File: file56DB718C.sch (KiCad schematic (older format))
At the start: 1 part, among them U4 SX1276

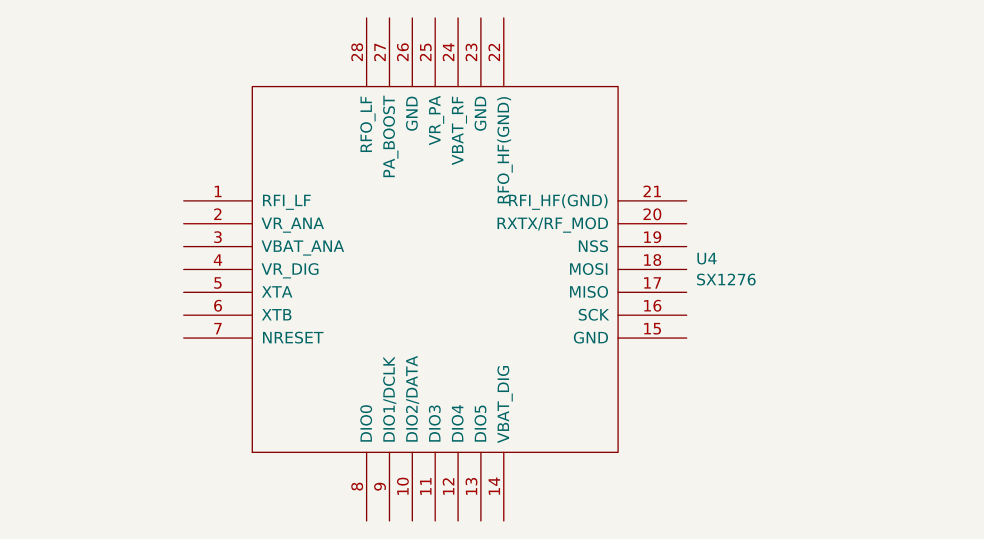
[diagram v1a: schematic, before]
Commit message: started layout, completed schematic
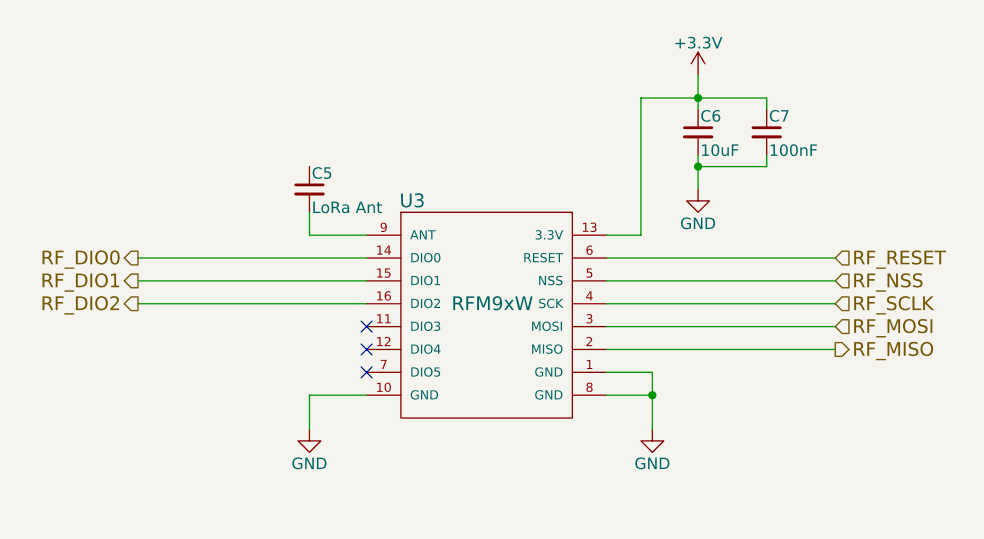
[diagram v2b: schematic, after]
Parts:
- removed U4: SX1276, Housings_DFN_QFN:QFN-28-1EP_6x6mm_Pitch0.65mm, symbol SX1276
- added C5: LoRa Ant, symbol C_Small
- added C6: 10uF, symbol C_Small
- added C7: 100nF, symbol C_Small
- added U3: RFM9xW, RocketScreamKicadLibrary:RFM9xW, symbol RFM9xW
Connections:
- new net: C5.2, U3.9 (ANT)
- new net +3V3: C6.1, C7.1, U3.13 (3.3V)
- new net GND: C6.2, C7.2, U3.1 (GND), U3.10 (GND), U3.8 (GND)
- new net RF_DIO0: U3.14 (DIO0)
- new net RF_DIO1: U3.15 (DIO1)
- new net RF_DIO2: U3.16 (DIO2)
- new net RF_MISO: U3.2 (MISO)
- new net RF_MOSI: U3.3 (MOSI)
- new net RF_NSS: U3.5 (NSS)
- new net RF_RESET: U3.6 (RESET)
- new net RF_SCLK: U3.4 (SCK)
- no-connect marks 0 -> 3
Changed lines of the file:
@@
 LIBS:mpu-9250
 LIBS:SAMD21E17A
+LIBS:miniultrapro
+LIBS:texas-instruments
 LIBS:lorawan_gps-cache
 EELAYER 25 0
@@
 $Descr A4 11693 8268
 encoding utf-8
-Sheet 5 7
+Sheet 4 7
 Title ""
 Date ""
@@
 $EndDescr
 $Comp
-L SX1276 U4
-U 1 1 56DB7573
-P 5400 3050
-F 0 "U4" H 6541 3096 50  0000 L CNN
-F 1 "SX1276" H 6541 3004 50  0000 L CNN
-F 2 "Housings_DFN_QFN:QFN-28-1EP_6x6mm_Pitch0.65mm" H 5400 3050 50  0001 C CNN
-F 3 "DOCUMENTATION" H 5400 3050 50  0001 C CNN
-	1    5400 3050
+L RFM9xW U3
+U 1 1 56EAE0A1
+P 5650 3250
+F 0 "U3" H 5300 3750 60  0000 C CNN
+F 1 "RFM9xW" H 5650 3300 60  0000 C CNN
+F 2 "RocketScreamKicadLibrary:RFM9xW" H 5650 2750 60  0001 C CNN
+F 3 "" H 5650 3550 60  0000 C CNN
+	1    5650 3250
 	1    0    0    -1
 $EndComp
+NoConn ~ 5100 3300
+NoConn ~ 5100 3400
+NoConn ~ 5100 3500
+$Comp
+L GND #PWR8
+U 1 1 56EAE13D
+P 4850 3750
+F 0 "#PWR8" H 4850 3500 50  0001 C CNN
+F 1 "GND" H 4850 3600 50  0000 C CNN
+F 2 "" H 4850 3750 50  0000 C CNN
+F 3 "" H 4850 3750 50  0000 C CNN
+	1    4850 3750
+	1    0    0    -1
+$EndComp
+$Comp
+L GND #PWR9
+U 1 1 56EAE153
+P 6350 3750
+F 0 "#PWR9" H 6350 3500 50  0001 C CNN
+F 1 "GND" H 6350 3600 50  0000 C CNN
+F 2 "" H 6350 3750 50  0000 C CNN
+F 3 "" H 6350 3750 50  0000 C CNN
+	1    6350 3750
+	1    0    0    -1
+$EndComp
+Wire Wire Line
+	6150 3500 6350 3500
+Wire Wire Line
+	6350 3500 6350 3750
+Wire Wire Line
+	6150 3600 6350 3600
+Connection ~ 6350 3600
+Wire Wire Line
+	4850 3750 4850 3600
+Wire Wire Line
+	4850 3600 5100 3600
+$Comp
+L +3.3V #PWR10
+U 1 1 56EAE17D
+P 6550 2200
+F 0 "#PWR10" H 6550 2050 50  0001 C CNN
+F 1 "+3.3V" H 6550 2340 50  0000 C CNN
+F 2 "" H 6550 2200 50  0000 C CNN
+F 3 "" H 6550 2200 50  0000 C CNN
+	1    6550 2200
+	1    0    0    -1
+$EndComp
+$Comp
+L C_Small C6
+U 1 1 56EAE19B
+P 6550 2450
+F 0 "C6" H 6560 2520 50  0000 L CNN
+F 1 "10uF" H 6560 2370 50  0000 L CNN
+F 2 "" H 6550 2450 50  0000 C CNN
+F 3 "" H 6550 2450 50  0000 C CNN
+	1    6550 2450
+	1    0    0    -1
+$EndComp
+$Comp
+L C_Small C7
+U 1 1 56EAE1DC
+P 6850 2450
+F 0 "C7" H 6860 2520 50  0000 L CNN
+F 1 "100nF" H 6860 2370 50  0000 L CNN
+F 2 "" H 6850 2450 50  0000 C CNN
+F 3 "" H 6850 2450 50  0000 C CNN
+	1    6850 2450
+	1    0    0    -1
+$EndComp
+Wire Wire Line
+	6150 2900 6300 2900
+Wire Wire Line
+	6300 2900 6300 2300
+Wire Wire Line
+	6300 2300 6850 2300
+Wire Wire Line
+	6850 2300 6850 2350
+Wire Wire Line
+	6550 2200 6550 2350
+Connection ~ 6550 2300
+$Comp
+L GND #PWR11
+U 1 1 56EAE25E
+P 6550 2700
+F 0 "#PWR11" H 6550 2450 50  0001 C CNN
+F 1 "GND" H 6550 2550 50  0000 C CNN
+F 2 "" H 6550 2700 50  0000 C CNN
+F 3 "" H 6550 2700 50  0000 C CNN
+	1    6550 2700
+	1    0    0    -1
+$EndComp
+Wire Wire Line
+	6550 2700 6550 2550
+Wire Wire Line
+	6550 2600 6850 2600
+Wire Wire Line
+	6850 2600 6850 2550
+Connection ~ 6550 2600
+Wire Wire Line
+	6150 3000 7150 3000
+Wire Wire Line
+	6150 3100 7150 3100
+Wire Wire Line
+	6150 3200 7150 3200
+Wire Wire Line
+	6150 3300 7150 3300
+Wire Wire Line
+	6150 3400 7150 3400
+Wire Wire Line
+	5100 3000 4100 3000
+Wire Wire Line
+	4100 3100 5100 3100
+Wire Wire Line
+	5100 3200 4100 3200
+Text HLabel 7150 3000 2    60   Input ~ 0
+RF_RESET
+Text HLabel 7150 3100 2    60   Input ~ 0
+RF_NSS
+Text HLabel 7150 3200 2    60   Input ~ 0
+RF_SCLK
+Text HLabel 7150 3300 2    60   Input ~ 0
+RF_MOSI
+Text HLabel 7150 3400 2    60   Output ~ 0
+RF_MISO
+Text HLabel 4100 3000 0    60   Output ~ 0
+RF_DIO0
+Text HLabel 4100 3100 0    60   Output ~ 0
+RF_DIO1
+Text HLabel 4100 3200 0    60   Output ~ 0
+RF_DIO2
+$Comp
+L C_Small C5
+U 1 1 56EBF9F4
+P 4850 2700
+F 0 "C5" H 4860 2770 50  0000 L CNN
+F 1 "LoRa Ant" H 4860 2620 50  0000 L CNN
+F 2 "" H 4850 2700 50  0000 C CNN
+F 3 "" H 4850 2700 50  0000 C CNN
+	1    4850 2700
+	1    0    0    -1
+$EndComp
+Wire Wire Line
+	4850 2900 5100 2900
+Wire Wire Line
+	4850 2900 4850 2800
 $EndSCHEMATC
